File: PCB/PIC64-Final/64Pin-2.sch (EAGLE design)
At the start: 172 parts, among them IC1 , IC2 , IC3 , IC4 , J1 84952-4, Q1 , Q2 IRF540, Q3 IRF540, Q4 IRF540, U1 LM5114BMFX/S7003094SOT26-GATE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, U2 LM5114BMFX/S7003094SOT26-GATE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, U3 LM5114BMFX/S7003094SOT26-GATE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, X2 , X3 , X4 , X5 , X6 , X7 , X8 , X9 

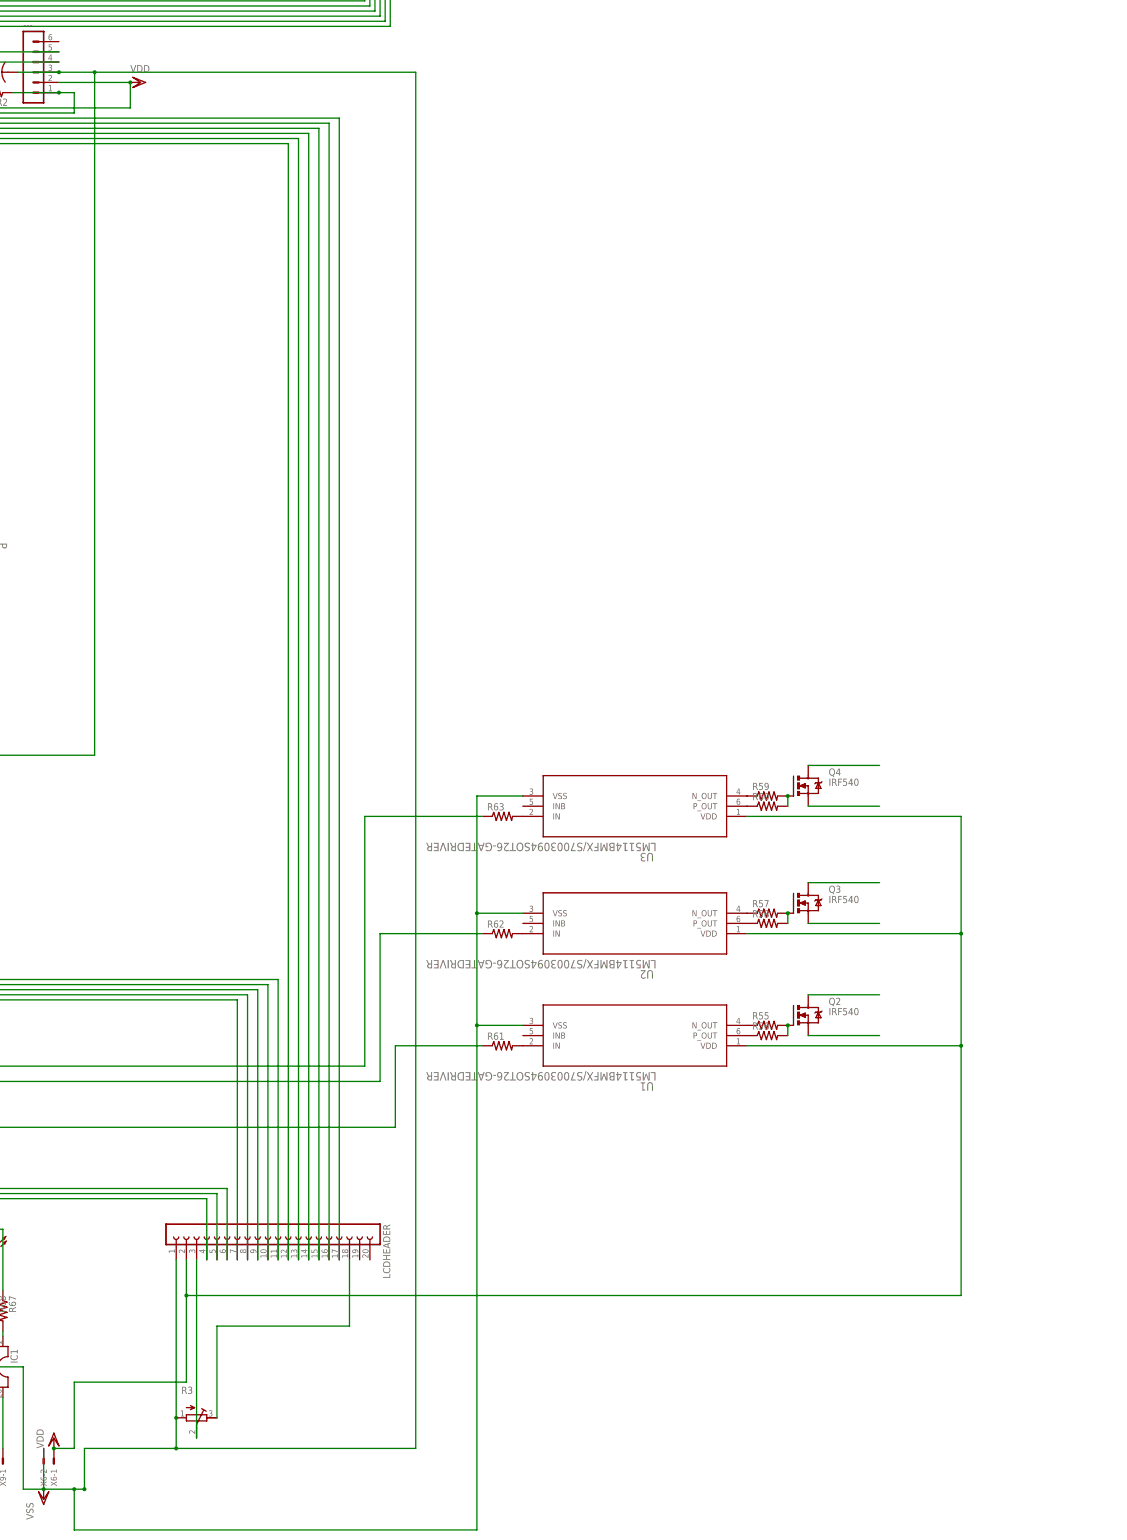
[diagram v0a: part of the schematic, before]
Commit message: D!!
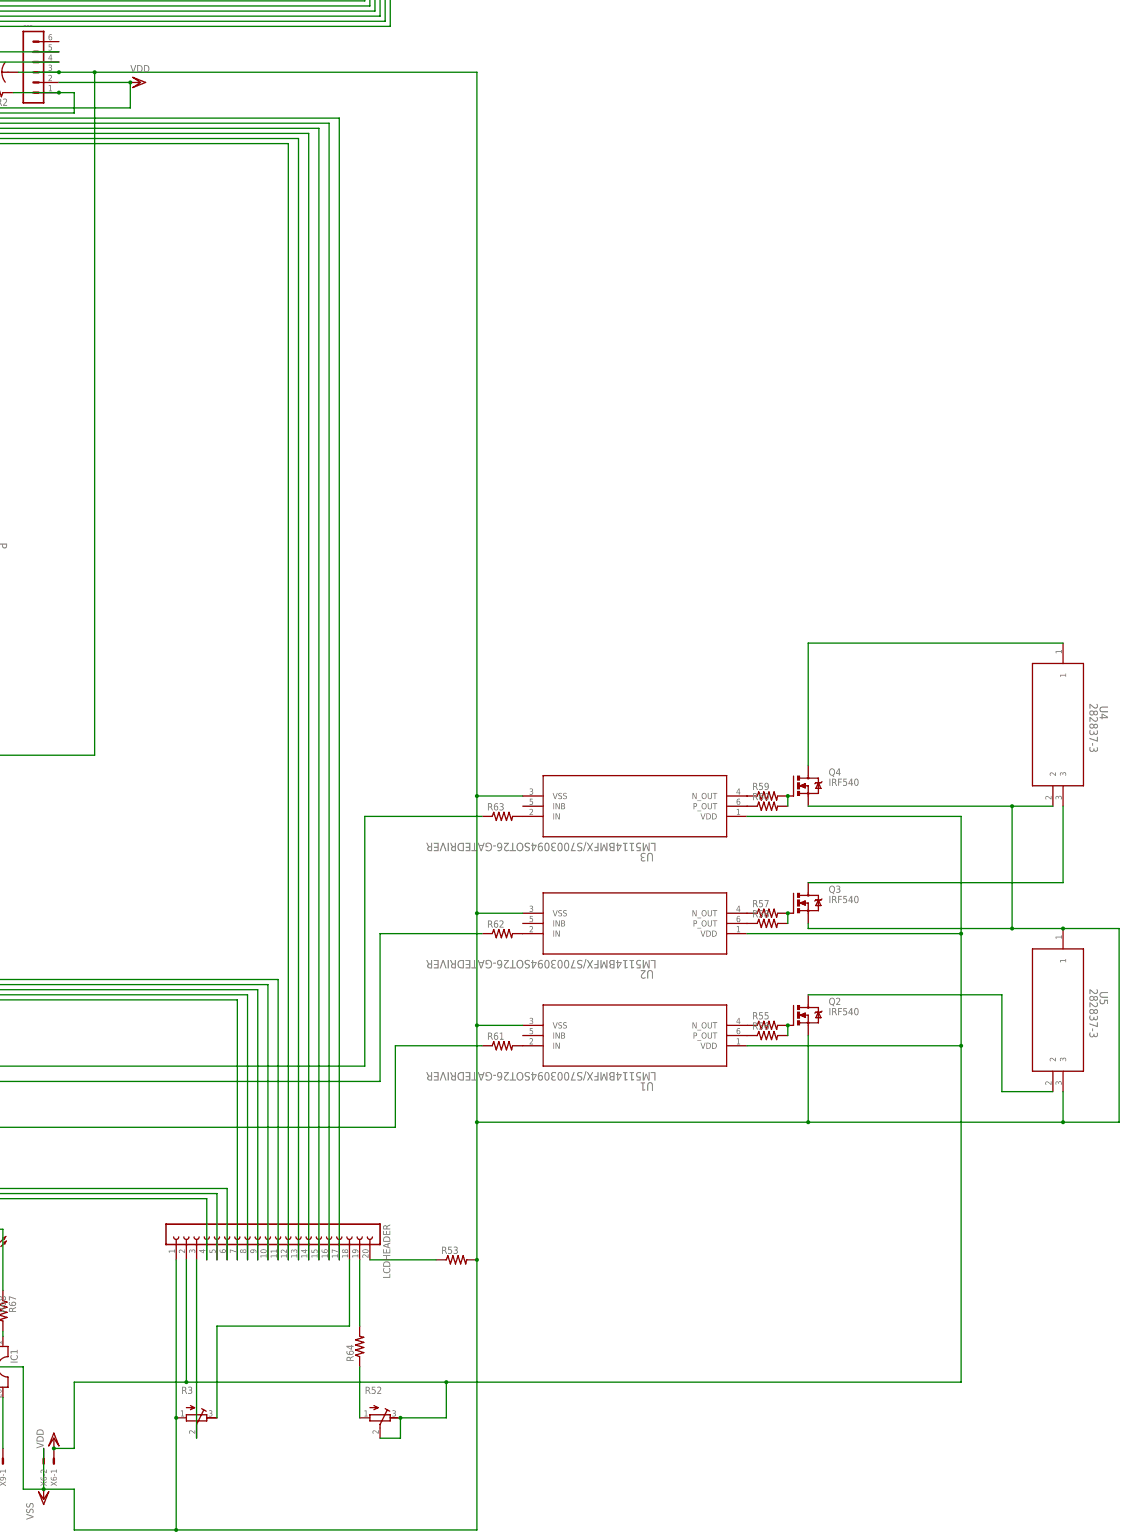
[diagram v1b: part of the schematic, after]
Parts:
- added R52: (no value), rcl:R-TRIMM3296W
- added R53, R64: (no value), resistor:R-US_R0603
- added U4, U5: 282837-3, 3-Pin-5.08:282837-3
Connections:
- new net N$46: Q4.D, U4.1
- new net N$65: Q3.D, U4.3
- new net N$74: Q2.D, U5.2
- net N$63: now also LCDHEADER.20, R53.1; no longer Q4.D
- net N$67: now also R52.A, R64.1; no longer Q3.D
- net N$75: now also LCDHEADER.19, R64.2; no longer Q2.D
- net VDD: now also R52.E, R52.S
- net VSS: now also R53.2, U4.2, U5.1, U5.3
